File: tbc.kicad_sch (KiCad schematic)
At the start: 0 parts

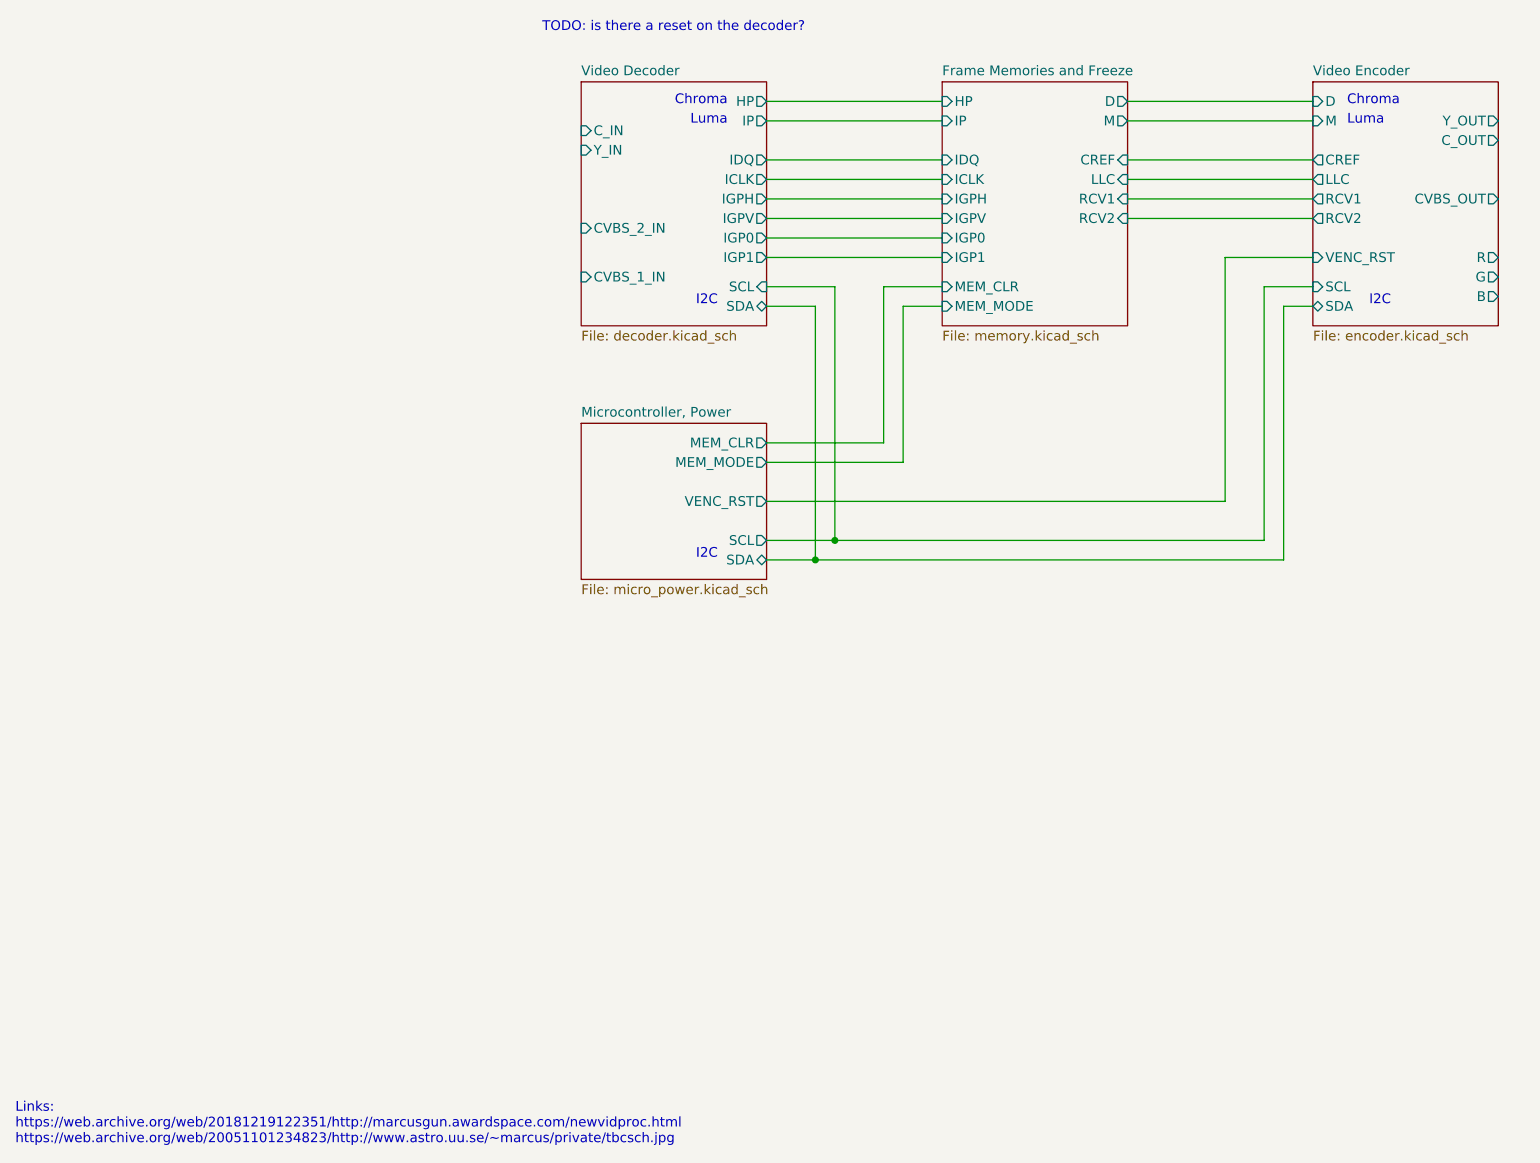
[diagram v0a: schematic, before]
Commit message: major progress with memory interfacing
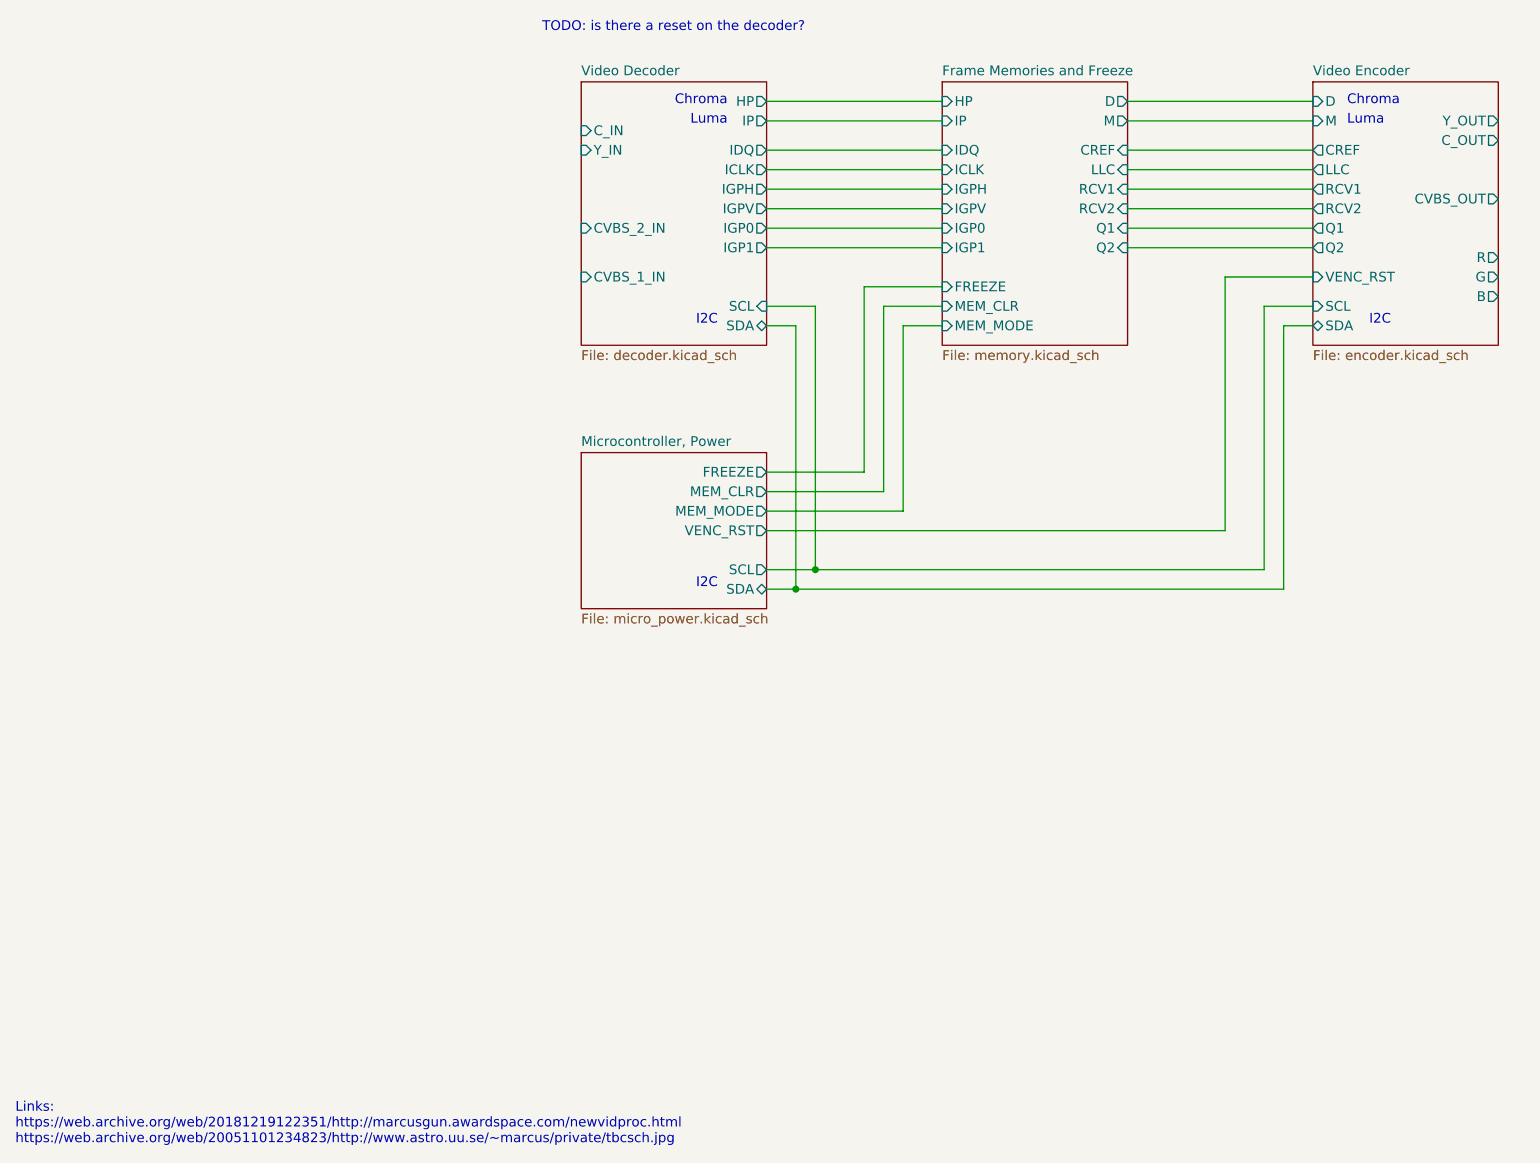
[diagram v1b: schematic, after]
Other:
- sheet Frame Memories and Freeze ports: added FREEZE, Q1, Q2; removed none
- sheet Microcontroller, Power ports: added FREEZE; removed none
- sheet Video Encoder ports: added Q1, Q2; removed none
